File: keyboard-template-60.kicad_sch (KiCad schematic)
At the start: 182 parts, among them J1 USB_C_Receptacle_USB2.0, J2 Conn_01x04_MountingPin, J3 AVR-ISP-6, J4 Conn_01x08_Pin, SW1 SW_Reset, U1 ATmega32U4-M, U2 SRV05-4, U3 TP_Sprintek_SK8707-01_Sensor, U6 AMS1117-3.3, Y1 8MHz

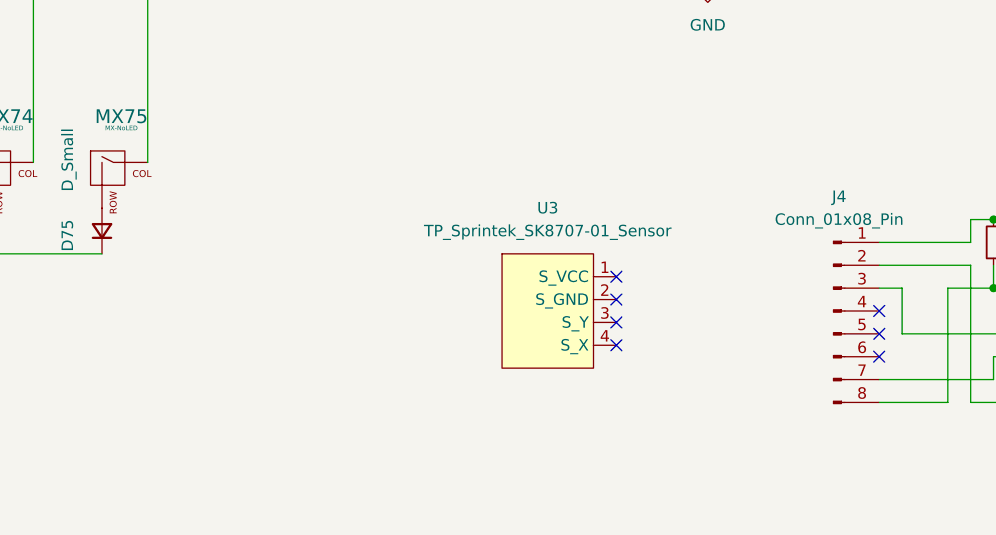
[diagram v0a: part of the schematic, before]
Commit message: Updates based on the 008
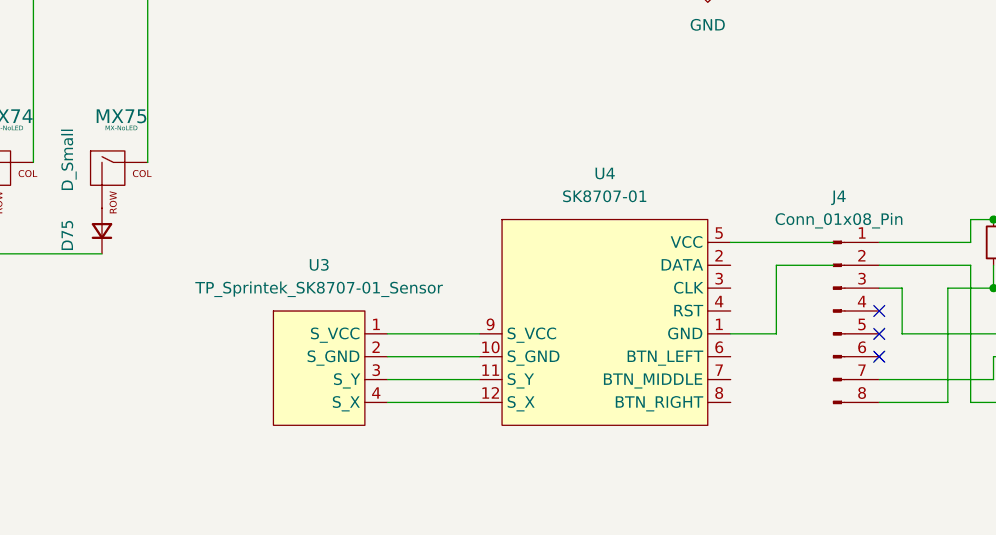
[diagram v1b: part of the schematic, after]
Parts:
- added U4: SK8707-01, ssbb_parts:TP_Sprintek_SK8707-01_reversible, symbol ssbb_parts:TP_Sprintek_SK8707–01
- U3: footprint ssbb_parts:TP_Sprintek_SK8707-01-005_Sensor_reversible -> ssbb_parts:TP_Sprintek_SK8707-01-008_Sensor
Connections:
- net at U3.1 (S_VCC): now also U4.9 (S_VCC)
- net at U3.2 (S_GND): now also U4.10 (S_GND)
- net at U3.3 (S_Y): now also U4.11 (S_Y)
- net at U3.4 (S_X): now also U4.12 (S_X)
- no-connect marks 12 -> 8
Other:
- moved on the sheet: U3
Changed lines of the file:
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@@
 	)
 	(no_connect
-		(at 287.02 219.71)
-	)
-	(no_connect
-		(at 287.02 217.17)
-	)
-	(no_connect
 		(at 358.14 173.99)
 	)
@@
 	)
 	(no_connect
-		(at 287.02 222.25)
-	)
-	(no_connect
 		(at 283.21 67.31)
 	)
@@
 	)
 	(no_connect
-		(at 287.02 224.79)
-	)
-	(no_connect
 		(at 316.23 226.06)
 	)
@@
 	(wire
 		(pts
+			(xy 261.62 231.14) (xy 271.78 231.14)
+		)
+		(stroke
+			(width 0)
+			(type default)
+		)
+	)
+	(wire
+		(pts
 			(xy 115.57 176.53) (xy 128.27 176.53)
 		)
@@
 	(wire
 		(pts
+			(xy 304.8 223.52) (xy 299.72 223.52)
+		)
+		(stroke
+			(width 0)
+			(type default)
+		)
+	)
+	(wire
+		(pts
 			(xy 234.95 166.37) (xy 234.95 204.47)
 		)
@@
 	(wire
 		(pts
+			(xy 261.62 223.52) (xy 271.78 223.52)
+		)
+		(stroke
+			(width 0)
+			(type default)
+		)
+	)
+	(wire
+		(pts
 			(xy 102.87 62.23) (xy 90.17 62.23)
 		)
@@
 	(wire
 		(pts
+			(xy 261.62 226.06) (xy 271.78 226.06)
+		)
+		(stroke
+			(width 0)
+			(type default)
+		)
+	)
+	(wire
+		(pts
 			(xy 294.64 44.45) (xy 298.45 44.45)
 		)
@@
 	(wire
 		(pts
+			(xy 311.15 215.9) (xy 304.8 215.9)
+		)
+		(stroke
+			(width 0)
+			(type default)
+		)
+	)
+	(wire
+		(pts
 			(xy 234.95 38.1) (xy 234.95 52.07)
 		)
@@
 	(wire
 		(pts
+			(xy 304.8 215.9) (xy 304.8 223.52)
+		)
+		(stroke
+			(width 0)
+			(type default)
+		)
+	)
+	(wire
+		(pts
 			(xy 321.31 49.53) (xy 321.31 52.07)
 		)
@@
 	(wire
 		(pts
+			(xy 299.72 213.36) (xy 311.15 213.36)
+		)
+		(stroke
+			(width 0)
+			(type default)
+		)
+	)
+	(wire
+		(pts
 			(xy 280.67 153.67) (xy 280.67 151.13)
 		)
@@
 	(wire
 		(pts
+			(xy 261.62 228.6) (xy 271.78 228.6)
+		)
+		(stroke
+			(width 0)
+			(type default)
+		)
+	)
+	(wire
+		(pts
 			(xy 323.85 218.44) (xy 323.85 231.14)
 		)
@@
 	(symbol
 		(lib_id "ssbb_parts:TP_Sprintek_SK8707-01_Sensor")
-		(at 279.4 220.98 0)
+		(at 254 227.33 0)
 		(unit 1)
 		(exclude_from_sim no)
@@
 		(fields_autoplaced yes)
 		(property "Reference" "U3"
-			(at 279.4 209.55 0)
+			(at 254 215.9 0)
 			(effects
 				(font
@@
 		)
 		(property "Value" "TP_Sprintek_SK8707-01_Sensor"
-			(at 279.4 212.09 0)
+			(at 254 218.44 0)
 			(effects
 				(font
@@
 			)
 		)
-		(property "Footprint" "ssbb_parts:TP_Sprintek_SK8707-01-005_Sensor_reversible"
-			(at 279.4 220.98 0)
+		(property "Footprint" "ssbb_parts:TP_Sprintek_SK8707-01-008_Sensor"
+			(at 254 227.33 0)
 			(effects
 				(font
@@
 		)
 		(property "Datasheet" ""
-			(at 279.4 220.98 0)
+			(at 254 227.33 0)
 			(effects
 				(font
@@
 		)
 		(property "Description" ""
-			(at 279.4 220.98 0)
+			(at 254 227.33 0)
 			(effects
 				(font
@@
 					(unit 1)
 				)
+			)
+		)
+	)
+	(symbol
+		(lib_id "ssbb_parts:TP_Sprintek_SK8707–01")
+		(at 285.75 222.25 0)
+		(unit 1)
+		(exclude_from_sim no)
+		(in_bom yes)
+		(on_board yes)
+		(dnp no)
+		(fields_autoplaced yes)
+		(property "Reference" "U4"
+			(at 285.75 205.74 0)
+			(effects
+				(font
+					(size 1.27 1.27)
+				)
+			)
+		)
+		(property "Value" "SK8707-01"
+			(at 285.75 208.28 0)
+			(effects
+				(font
+					(size 1.27 1.27)
+				)
+			)
+		)
+		(property "Footprint" "ssbb_parts:TP_Sprintek_SK8707-01_reversible"
+			(at 285.75 222.25 0)
+			(effects
+				(font
+					(size 1.27 1.27)
+				)
+				(hide yes)
+			)
+		)
+		(property "Datasheet" ""
+			(at 285.75 222.25 0)
+			(effects
+				(font
+					(size 1.27 1.27)
+				)
+				(hide yes)
+			)
+		)
+		(property "Description" ""
+			(at 285.75 222.25 0)
+			(effects
+				(font
+					(size 1.27 1.27)
+				)
+				(hide yes)
+			)
+		)
+		(pin "1"
+		)
+		(pin "4"
+		)
+		(pin "12"
+		)
+		(pin "6"
+		)
+		(pin "5"
+		)
+		(pin "2"
+		)
+		(pin "3"
+		)
+		(pin "11"
+		)
+		(pin "10"
+		)
+		(pin "9"
+		)
+		(pin "7"
+		)
+		(pin "8"
+		)
+		(instances
+			(project ""
+				(path "/b3baaebd-c99d-4218-99ba-d40a73031965"
+					(reference "U4")
+					(unit 1)
+				)
